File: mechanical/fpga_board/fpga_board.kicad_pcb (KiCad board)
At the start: 4 copper layers, 92 x 92 mm, 52 parts, among them J1 Conn_02x17_Odd_Even, J10 Conn_01x01, J2 Conn_02x17_Odd_Even, J3 Conn_02x17_Odd_Even, J4 Conn_02x17_Odd_Even, J5 Conn_02x17_Odd_Even, J6 jtag, J7 Conn_02x03_Odd_Even, J8 Conn_02x12_Odd_Even, J9 Conn_01x01, U1 XC6SLX16-FTG256, U2 SiT1602, U3 MIC5504-3.3YM5, U4 MIC5504-1.2YM5

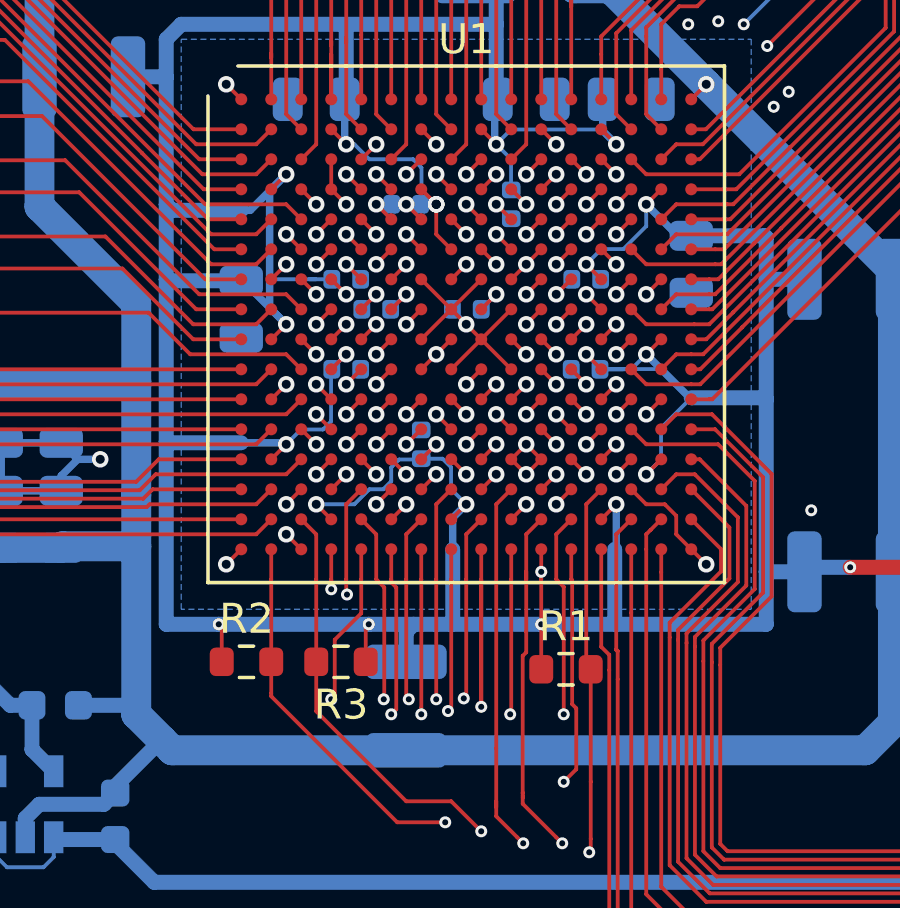
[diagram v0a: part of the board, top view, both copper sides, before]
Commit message: drc fixes
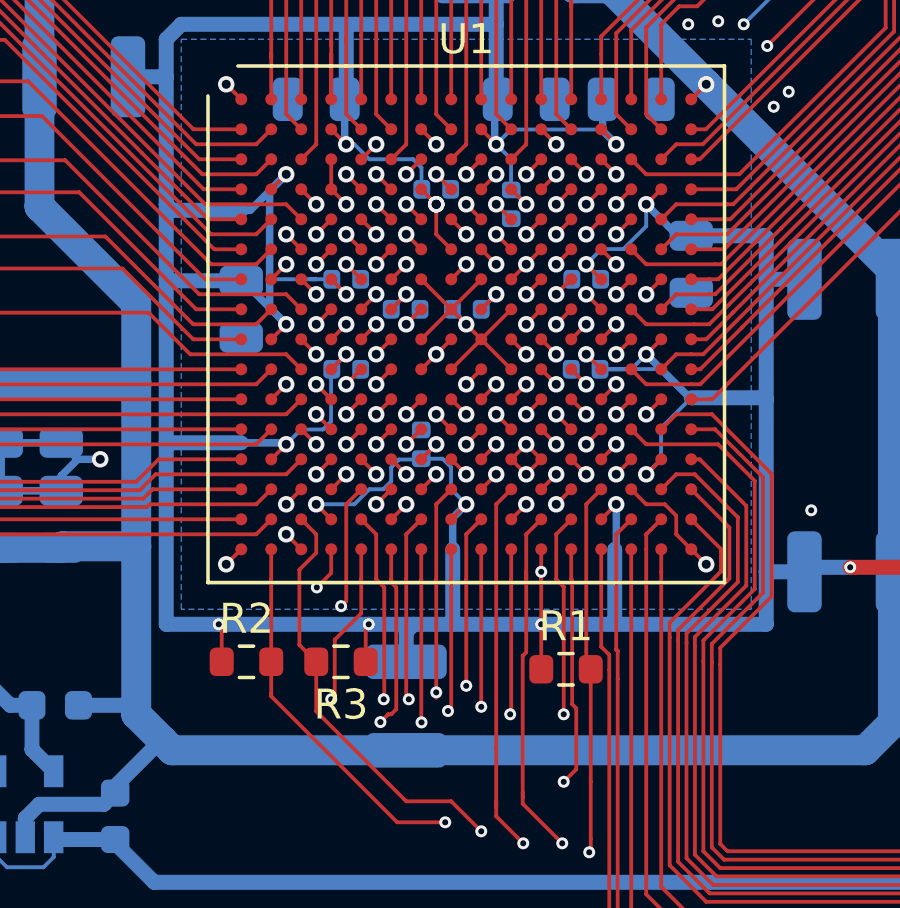
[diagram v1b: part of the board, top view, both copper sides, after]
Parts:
- moved C17 1.12 mm to (267.0, 199.2), turned to 0 degrees
- moved C18 0.98 mm to (266.0, 203.2), turned to 0 degrees
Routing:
- net /T9+5: track 22.0 -> 16.8 mm
- net /T12-5: track 19.4 -> 17.4 mm
- net /T15-5: track 25.5 -> 23.6 mm
- net /T10+5: track 20.0 -> 18.2 mm
- net /T16-5: track 22.7 -> 21.2 mm
- net /T13+5: track 20.9 -> 19.6 mm
- net /T1-4: track 69.3 -> 68.7 mm
- net /T11-5: track 20.9 -> 21.6 mm
- net /T5+4: track 95.0 -> 95.6 mm
